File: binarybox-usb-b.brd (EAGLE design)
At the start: 142.2 x 91.4 mm, 29 parts, among them IC2 MAX7219CNG, X1 USBPTH

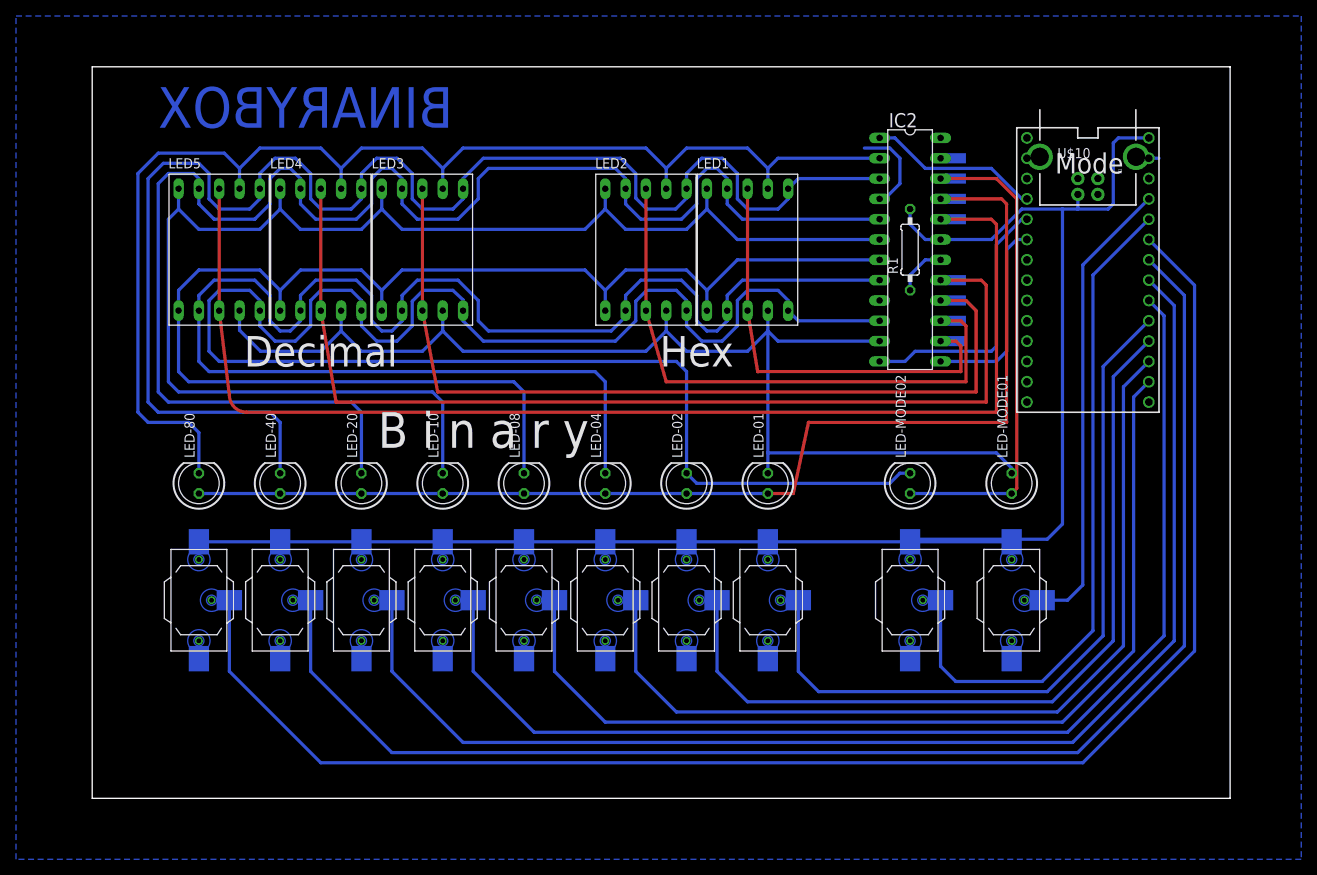
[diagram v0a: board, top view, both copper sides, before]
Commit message: cleaned up usb board and arduino sketch
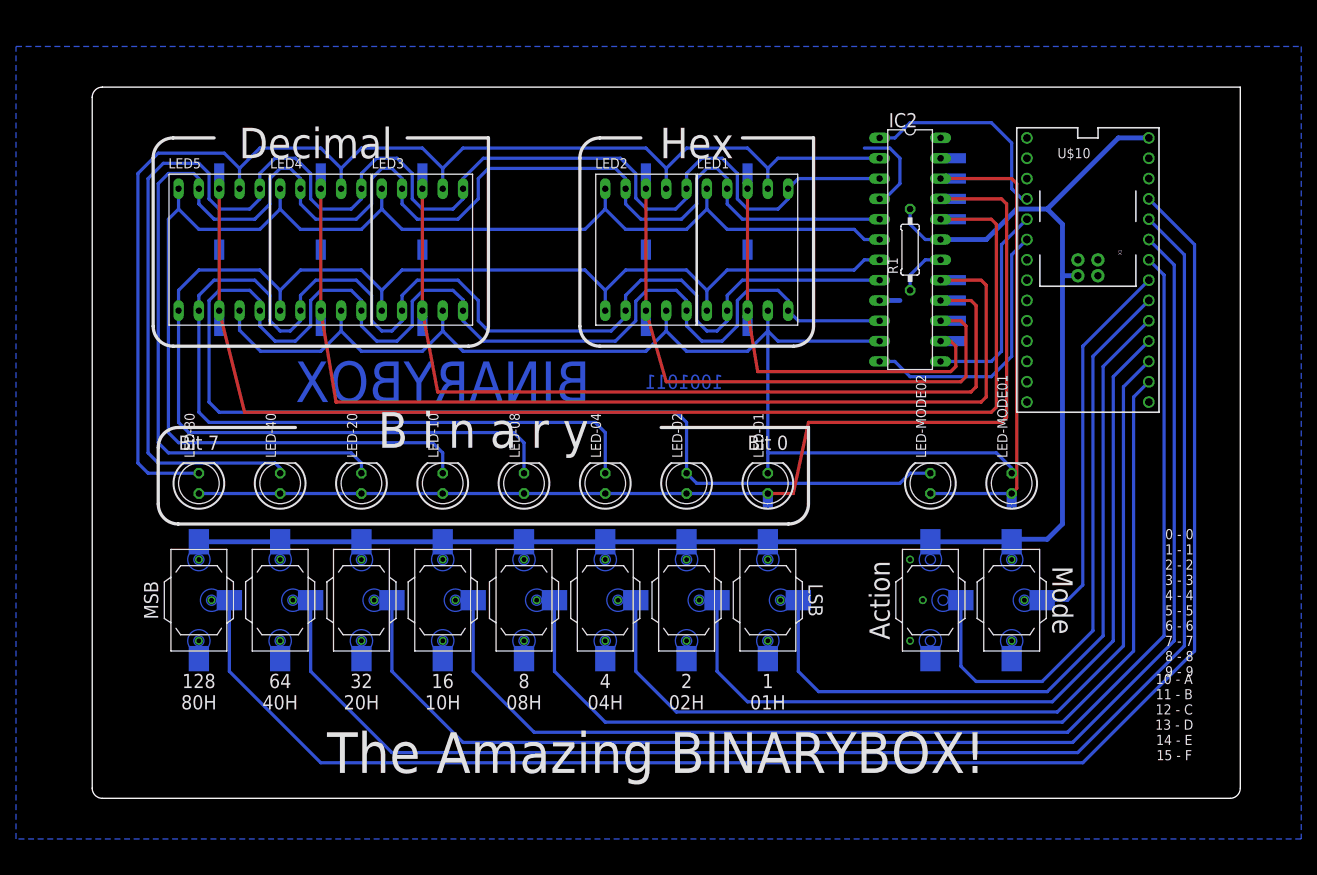
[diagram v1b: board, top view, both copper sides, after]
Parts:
- moved X1 10.2 mm to (124.5, 67.3)
- moved LED-MODE02 2.54 mm to (104.8, 39.4)
- moved U$13 2.54 mm to (104.8, 24.8)
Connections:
- net CLK: now also U$10.3; no longer U$10.4
- net INP10: now also U$10.20/A6; no longer U$10.18/A4
- net INP20: now also U$10.21/A7; no longer U$10.19/A5
- net INP40: now also U$10.22/A8; no longer U$10.20/A6
- net INP80: now also U$10.23/A9; no longer U$10.21/A7
- net LOAD: now also U$10.4; no longer U$10.3
- net MODE01: now also U$10.19/A5; no longer U$10.23/A9
- net MODE02: now also U$10.18/A4; no longer U$10.22/A8
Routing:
- net VCC: track 205.2 -> 189.0 mm
- net MODE02: track 85.1 -> 72.4 mm
- net MODE01: track 57.5 -> 47.4 mm
- net INP80: track 193.9 -> 198.9 mm
- net INP40: track 177.9 -> 183.0 mm
- net INP10: track 146.1 -> 151.2 mm
- net INP20: track 162.0 -> 167.1 mm
- net DIN: track 21.6 -> 26.5 mm
- net SEGDP: track 230.5 -> 233.1 mm
- net CA1: track 54.3 -> 52.7 mm
- net CA7: track 60.4 -> 58.9 mm
- net CLK: track 24.5 -> 26.0 mm
- net GND: track 12.7 -> 14.0 mm
- net SEGA: track 159.8 -> 160.5 mm
- net CA5: track 153.4 -> 152.7 mm
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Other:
- board size 142.2 x 91.4 mm -> 143.5 x 88.9 mm
- board text added: "0 - 0 1 - 1 2 - 2 3 - 3 4 - 4 5 - 5 6 - 6 7 - 7 8 - 8 9 - 9"
- board text added: "1 01H"
- board text added: "10 - A 11 - B 12 - C 13 - D 14 - E 15 - F"
- board text added: "1001011"
- board text added: "128 80H"
- board text added: "16 10H"
- board text added: "2 02H"
- board text added: "32 20H"
- board text added: "4 04H"
- board text added: "64 40H"
- board text added: "8 08H"
- board text added: "Action"
- board text added: "Bit 0"
- board text added: "Bit 7"
- board text added: "LSB"
- board text added: "MSB"
- board text added: "The Amazing BINARYBOX!"
